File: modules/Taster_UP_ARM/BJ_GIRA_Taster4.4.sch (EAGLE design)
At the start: 68 parts, among them IC1 LPC1115, IC100 BD9G101, T1 BC856, T2 BCP52, T3 BC847

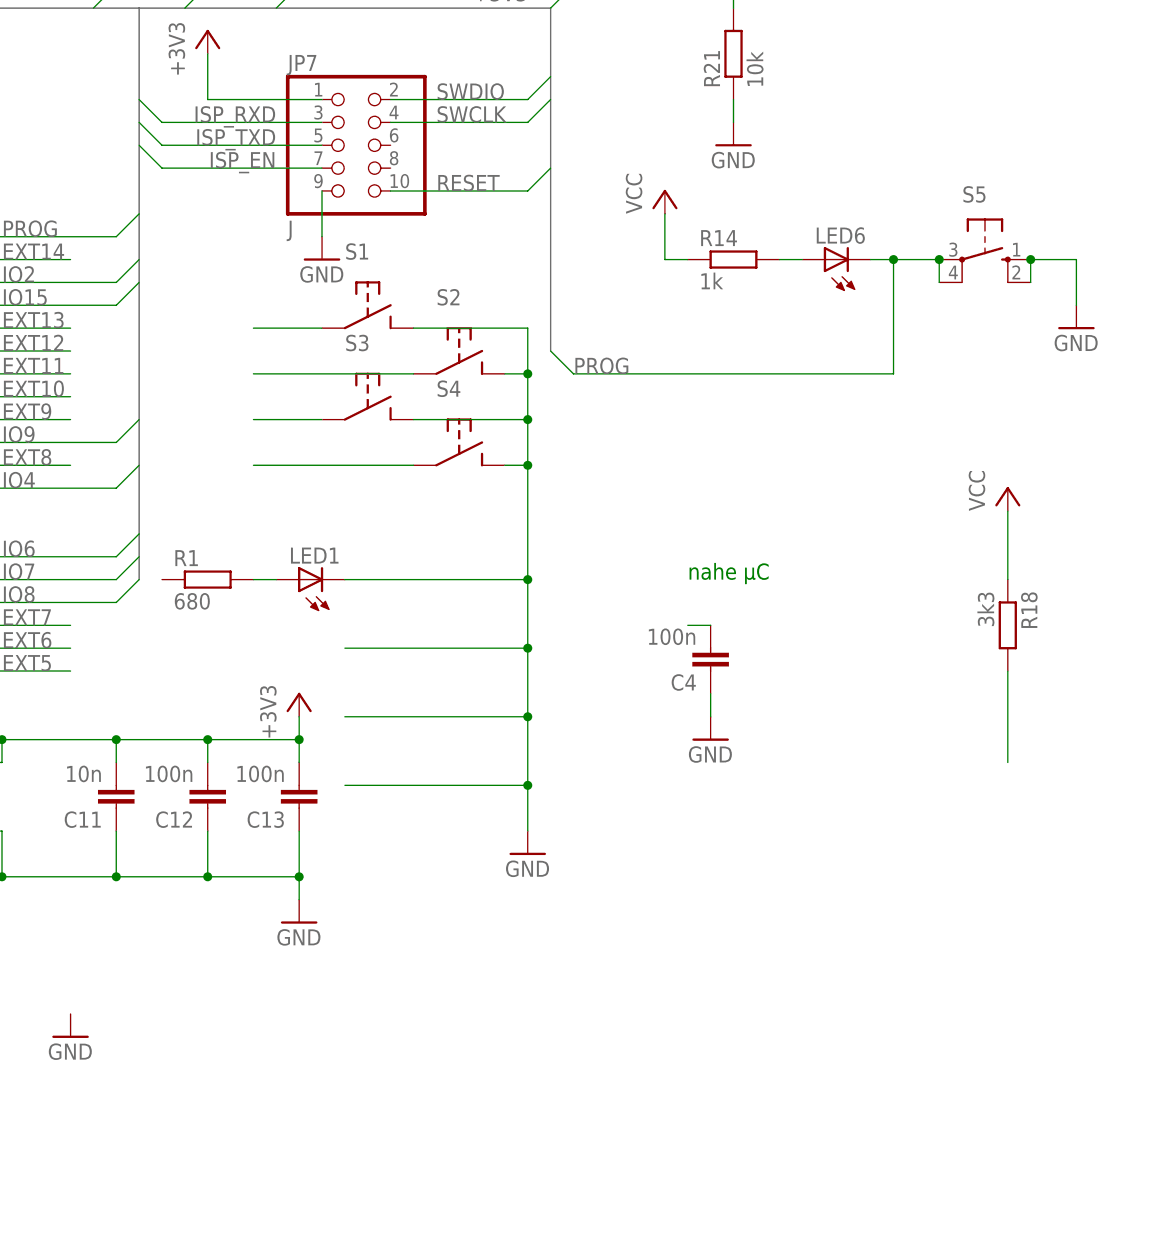
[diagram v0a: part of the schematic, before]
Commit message: naechster Vorschlag
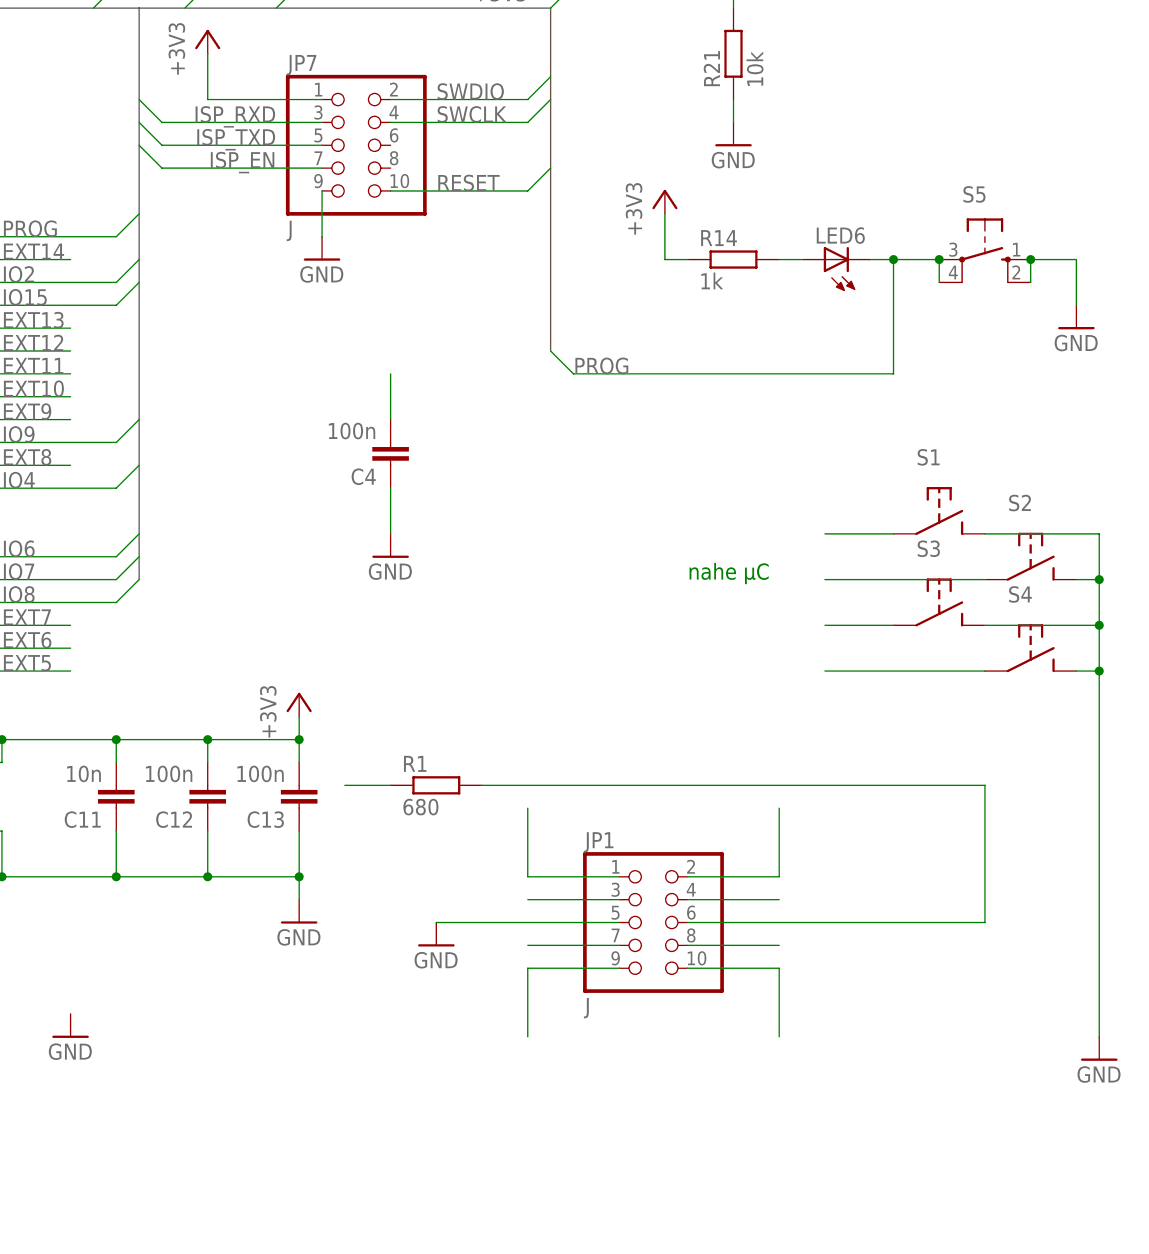
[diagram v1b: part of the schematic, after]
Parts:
- removed LED1: (no value), led:LED3MM
- removed R18: 3k3, rcl:R-EU_R1206
- added JP1: J, pinhead-2:PINHD-2X05_2.00
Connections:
- removed net INT0: R18.2
- removed net VCC: R14.1, R18.1
- new net N$15: JP1.3
- new net N$20: JP1.4
- new net N$21: JP1.8
- new net N$22: JP1.7
- net +3V3: now also R14.1
- net EXT11: now also JP1.10, R1.1
- net EXT14: now also JP1.1
- net EXT7: now also S1.1
- net GND: now also JP1.5; no longer LED1.C
- net IO15: now also JP1.9
- net IO2: now also JP1.2; no longer S1.1
- net N$8: now also JP1.6; no longer LED1.A
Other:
- moved on the sheet: C4, R1, S1, S2, S3, S4

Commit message: vorschlag Erweiterungsstecker
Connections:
- removed net N$15: JP1.3
- removed net N$20: JP1.4
- removed net N$21: JP1.8
- removed net N$22: JP1.7
- net +3V3: now also JP1.4
- net EXT5: now also JP1.7
- net EXT6: now also JP1.8
- net IO4: now also JP1.3
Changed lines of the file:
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@@
 <label x="149.86" y="205.74" size="1.778" layer="95"/>
+</segment>
+<segment>
+<pinref part="JP1" gate="A" pin="3"/>
+<wire x1="218.44" y1="160.02" x2="208.28" y2="160.02" width="0.1524" layer="91"/>
 </segment>
 </net>
@@
 <pinref part="P+2" gate="G$1" pin="+3V3"/>
 </segment>
+<segment>
+<pinref part="JP1" gate="A" pin="4"/>
+<wire x1="226.06" y1="160.02" x2="236.22" y2="160.02" width="0.1524" layer="91"/>
+</segment>
 </net>
 <net name="IO16" class="0">
@@
 <label x="149.86" y="187.96" size="1.778" layer="95"/>
 </segment>
+<segment>
+<pinref part="JP1" gate="A" pin="8"/>
+<wire x1="226.06" y1="154.94" x2="236.22" y2="154.94" width="0.1524" layer="91"/>
+</segment>
 </net>
 <net name="EXT5" class="0">
@@
 <wire x1="147.32" y1="185.42" x2="157.48" y2="185.42" width="0.1524" layer="91"/>
 <label x="149.86" y="185.42" size="1.778" layer="95"/>
+</segment>
+<segment>
+<pinref part="JP1" gate="A" pin="7"/>
+<wire x1="218.44" y1="154.94" x2="208.28" y2="154.94" width="0.1524" layer="91"/>
 </segment>
 </net>
@@
 </segment>
 </net>
-<net name="N$15" class="0">
-<segment>
-<pinref part="JP1" gate="A" pin="3"/>
-<wire x1="218.44" y1="160.02" x2="208.28" y2="160.02" width="0.1524" layer="91"/>
-</segment>
-</net>
-<net name="N$20" class="0">
-<segment>
-<pinref part="JP1" gate="A" pin="4"/>
-<wire x1="226.06" y1="160.02" x2="236.22" y2="160.02" width="0.1524" layer="91"/>
-</segment>
-</net>
-<net name="N$21" class="0">
-<segment>
-<pinref part="JP1" gate="A" pin="8"/>
-<wire x1="226.06" y1="154.94" x2="236.22" y2="154.94" width="0.1524" layer="91"/>
-</segment>
-</net>
-<net name="N$22" class="0">
-<segment>
-<pinref part="JP1" gate="A" pin="7"/>
-<wire x1="218.44" y1="154.94" x2="208.28" y2="154.94" width="0.1524" layer="91"/>
-</segment>
-</net>
